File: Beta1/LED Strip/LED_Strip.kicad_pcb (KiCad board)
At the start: 2 copper layers, 163.2 x 8.9 mm, 100 parts, among them U0 APA102C, U1 APA102C, U10 APA102C, U11 APA102C, U12 APA102C, U13 APA102C, U14 APA102C, U15 APA102C, U2 APA102C, U3 APA102C, U4 APA102C, U5 APA102C, U6 APA102C, U7 APA102C, U8 APA102C, U9 APA102C

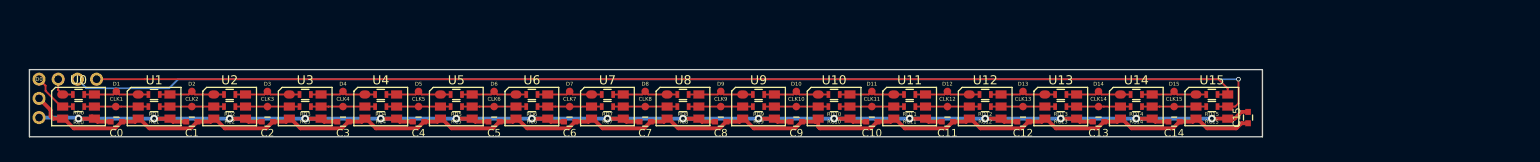
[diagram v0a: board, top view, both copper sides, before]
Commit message: Knob / LED Module WIP
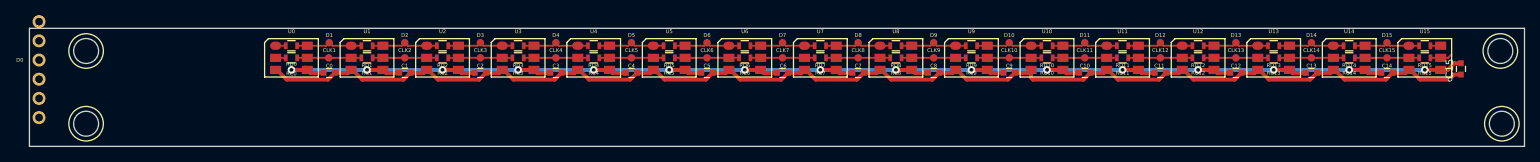
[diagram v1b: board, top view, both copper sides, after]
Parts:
- added REF**: 1pin, Connect:1pin, F.Cu at (7.50, -12.6)
- added REF**: 1pin, Connect:1pin, F.Cu at (7.50, -3.00)
- added REF**: 1pin, Connect:1pin, F.Cu at (194.7, -12.6)
- added REF**: 1pin, Connect:1pin, F.Cu at (194.9, -3.00)
- moved C10 28.9 mm to (139.7, -9.72)
- moved C11 28.9 mm to (149.7, -9.72)
- moved C12 28.9 mm to (159.7, -9.72)
- moved C13 28.9 mm to (169.7, -9.72)
- moved C14 28.9 mm to (179.7, -9.72)
- moved C15 28.9 mm to (189.5, -10.3)
- moved C3 28.9 mm to (69.7, -9.72)
- moved C4 28.9 mm to (79.7, -9.72)
- moved C5 28.9 mm to (89.7, -9.72)
- moved C6 28.9 mm to (99.7, -9.72)
- moved C7 28.9 mm to (109.7, -9.72)
- moved C8 28.9 mm to (119.7, -9.72)
- moved C9 28.9 mm to (129.7, -9.72)
- moved CLK10 28.9 mm to (129.7, -11.7)
- moved CLK11 28.9 mm to (139.7, -11.7)
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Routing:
- net /CLK16: track 160.8 -> 2.95 mm, vias 1 -> 0
- net /D16: track 152.6 -> 1.54 mm
- net (no net): track 8.26 -> 0.00 mm
- net +5V: track 227.1 -> 222.1 mm
- net Net-(CLK0-Pad1): track 6.38 -> 1.54 mm
- net GND: track 179.6 -> 174.9 mm, vias 0 -> 1
- net Net-(D0-Pad1): track 3.61 -> 1.35 mm
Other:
- board size 163.2 x 8.9 mm -> 197.9 x 15.6 mm
